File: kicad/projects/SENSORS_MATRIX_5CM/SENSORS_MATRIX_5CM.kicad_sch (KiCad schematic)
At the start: 15 parts, among them J1 Conn_02x11_Odd_Even

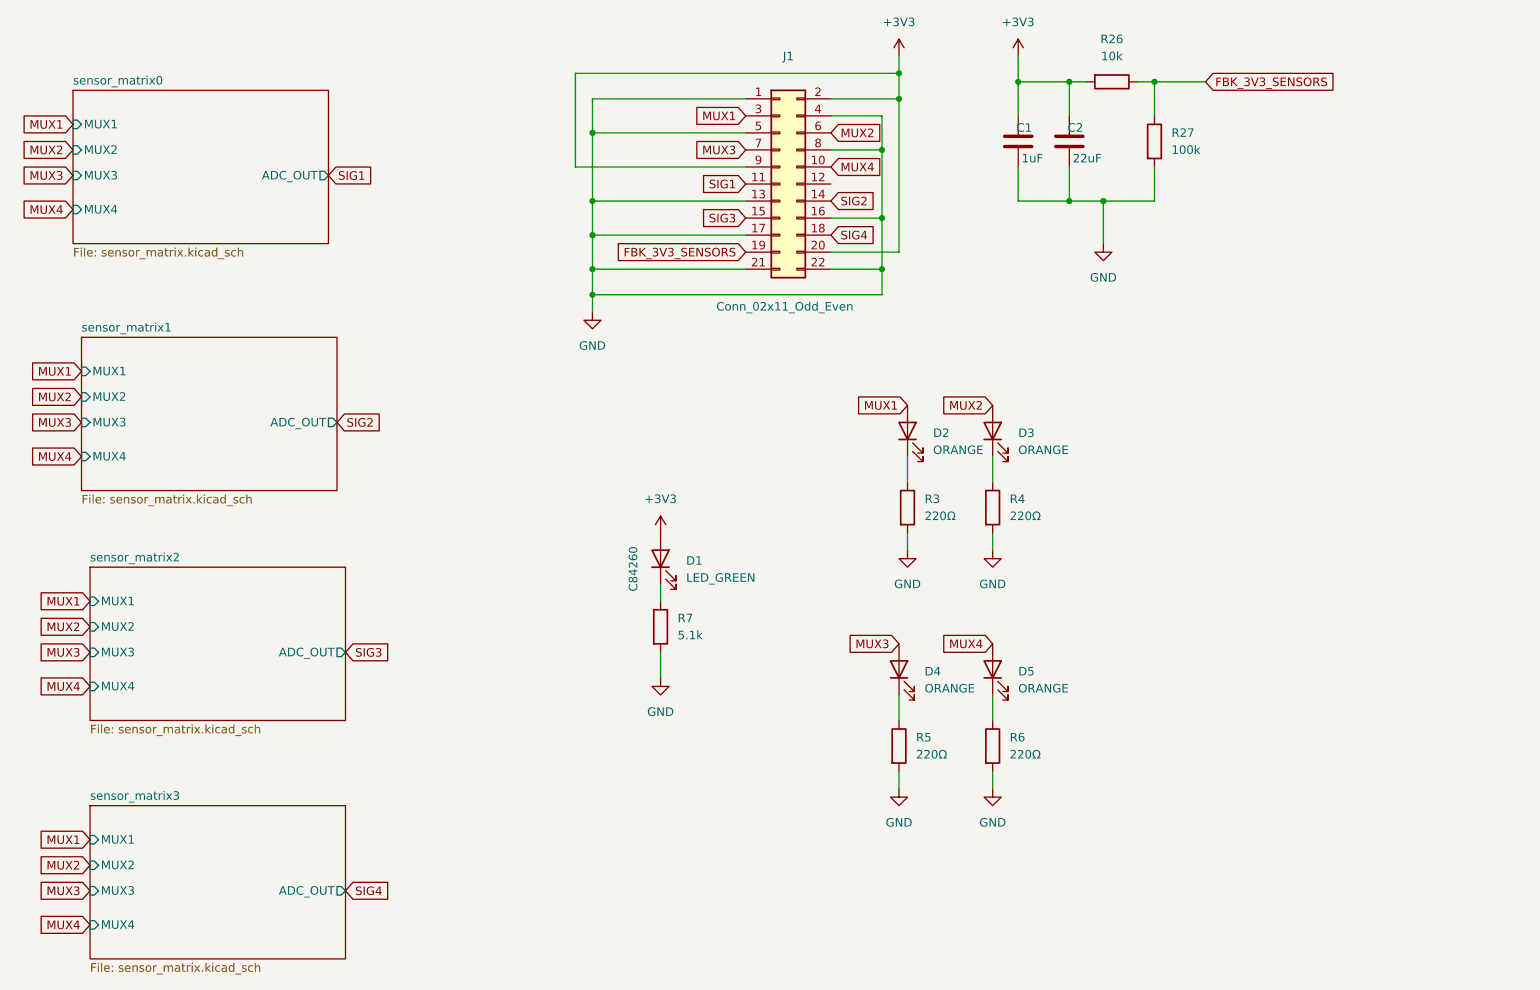
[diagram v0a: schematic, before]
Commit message: sensors board almost finished
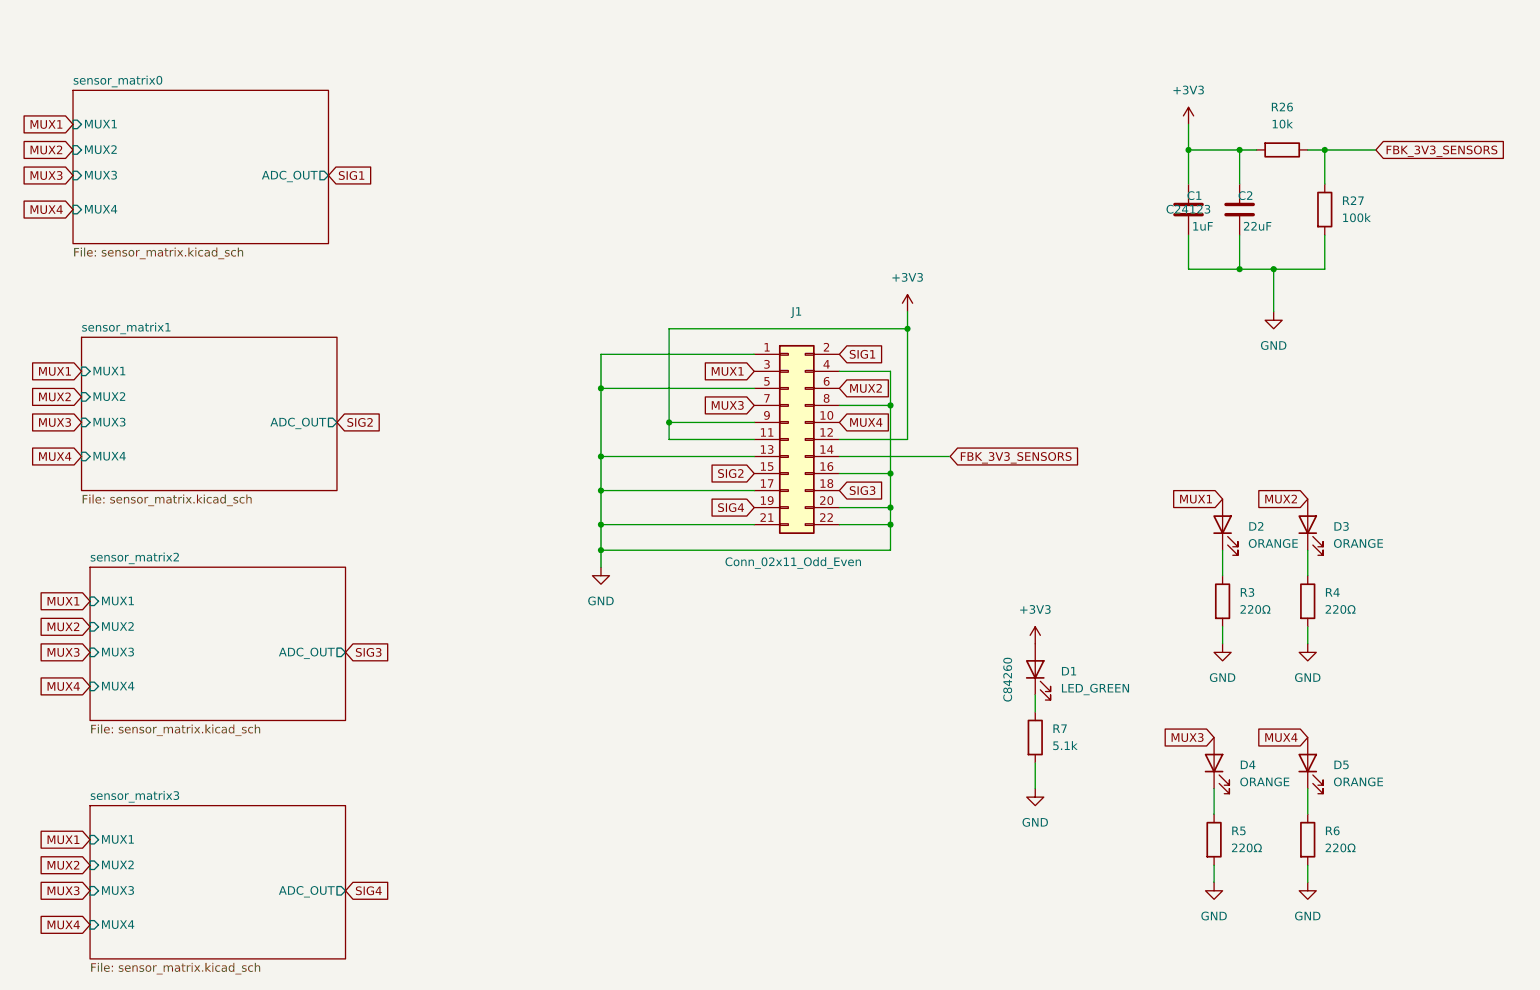
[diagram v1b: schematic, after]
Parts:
- C1: LCSC p/n (none) -> C24123
- C2: MP CL21A105KOFNNNE -> (none); shop https://www.lcsc.com/product-detail/Multilayer-Ceramic-Capa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 -> (none)
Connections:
- net +3V3: now also J1.11 (Pin_11), J1.12 (Pin_12); no longer J1.2 (Pin_2), J1.20 (Pin_20)
- net FBK_3V3_SENSORS: now also J1.14 (Pin_14); no longer J1.19 (Pin_19)
- net GND: now also J1.20 (Pin_20)
- net SIG1: now also J1.2 (Pin_2); no longer J1.11 (Pin_11)
- net SIG2: now also J1.15 (Pin_15); no longer J1.14 (Pin_14)
- net SIG3: now also J1.18 (Pin_18); no longer J1.15 (Pin_15)
- net SIG4: now also J1.19 (Pin_19); no longer J1.18 (Pin_18)
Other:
- moved on the sheet: C1, C2, D1, D2, D3, D4, D5, J1, R26, R27, R3, R4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
